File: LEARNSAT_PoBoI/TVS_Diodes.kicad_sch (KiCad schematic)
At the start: 4 parts

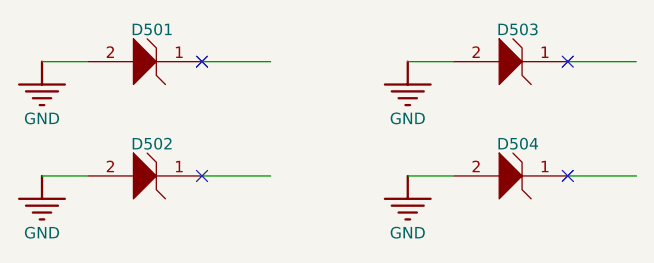
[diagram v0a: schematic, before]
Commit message: Add files via upload
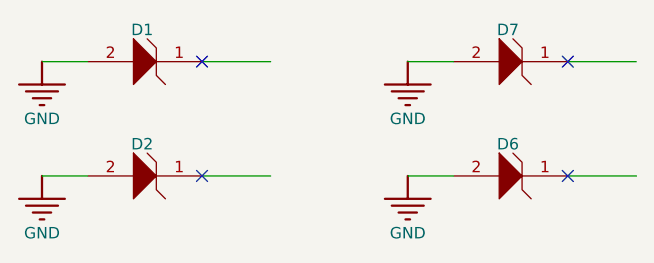
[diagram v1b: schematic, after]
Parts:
- D1: renamed from D501; footprint Diode_SMD:D_SOD-323 -> ONSC-SOD-323-2-477-02_V
- D2: renamed from D502; footprint Diode_SMD:D_SOD-323 -> ONSC-SOD-323-2-477-02_V
- D6: renamed from D504; footprint Diode_SMD:D_SOD-323 -> ONSC-SOD-323-2-477-02_V
- D7: renamed from D503; footprint Diode_SMD:D_SOD-323 -> ONSC-SOD-323-2-477-02_V
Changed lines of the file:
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@@
 		(on_board yes)
 		(dnp no)
-		(property "Reference" "#PWR0502"
+		(property "Reference" "#PWR?"
 			(at 58.42 111.76 0)
 			(effects
@@
 			(project ""
 				(path "/31302da5-a970-4b2b-aa05-afcd06cb9d09/9724113b-8f83-448f-99ae-c96db2fb53ca"
-					(reference "#PWR0502")
+					(reference "#PWR?")
 					(unit 1)
 				)
@@
 		(on_board yes)
 		(dnp no)
-		(property "Reference" "D503"
+		(property "Reference" "D7"
 			(at 108.966 96.266 0)
 			(effects
@@
 			)
 		)
-		(property "Footprint" "Diode_SMD:D_SOD-323"
+		(property "Footprint" "ONSC-SOD-323-2-477-02_V"
 			(at 111.76 101.6 0)
 			(effects
@@
 			(project ""
 				(path "/31302da5-a970-4b2b-aa05-afcd06cb9d09/9724113b-8f83-448f-99ae-c96db2fb53ca"
-					(reference "D503")
+					(reference "D7")
 					(unit 1)
 				)
@@
 		(on_board yes)
 		(dnp no)
-		(property "Reference" "#PWR0503"
+		(property "Reference" "#PWR?"
 			(at 99.06 99.06 0)
 			(effects
@@
 			(project ""
 				(path "/31302da5-a970-4b2b-aa05-afcd06cb9d09/9724113b-8f83-448f-99ae-c96db2fb53ca"
-					(reference "#PWR0503")
+					(reference "#PWR?")
 					(unit 1)
 				)
@@
 		(on_board yes)
 		(dnp no)
-		(property "Reference" "#PWR0504"
+		(property "Reference" "#PWR?"
 			(at 99.06 111.76 0)
 			(effects
@@
 			(project ""
 				(path "/31302da5-a970-4b2b-aa05-afcd06cb9d09/9724113b-8f83-448f-99ae-c96db2fb53ca"
-					(reference "#PWR0504")
+					(reference "#PWR?")
 					(unit 1)
 				)
@@
 		(on_board yes)
 		(dnp no)
-		(property "Reference" "D504"
+		(property "Reference" "D6"
 			(at 108.966 108.966 0)
 			(effects
@@
 			)
 		)
-		(property "Footprint" "Diode_SMD:D_SOD-323"
+		(property "Footprint" "ONSC-SOD-323-2-477-02_V"
 			(at 111.76 114.3 0)
 			(effects
@@
 			(project ""
 				(path "/31302da5-a970-4b2b-aa05-afcd06cb9d09/9724113b-8f83-448f-99ae-c96db2fb53ca"
-					(reference "D504")
+					(reference "D6")
 					(unit 1)
 				)
@@
 		(on_board yes)
 		(dnp no)
-		(property "Reference" "D501"
+		(property "Reference" "D1"
 			(at 68.326 96.266 0)
 			(effects
@@
 			)
 		)
-		(property "Footprint" "Diode_SMD:D_SOD-323"
+		(property "Footprint" "ONSC-SOD-323-2-477-02_V"
 			(at 71.12 101.6 0)
 			(effects
@@
 			(project ""
 				(path "/31302da5-a970-4b2b-aa05-afcd06cb9d09/9724113b-8f83-448f-99ae-c96db2fb53ca"
-					(reference "D501")
+					(reference "D1")
 					(unit 1)
 				)
@@
 		(on_board yes)
 		(dnp no)
-		(property "Reference" "D502"
+		(property "Reference" "D2"
 			(at 68.326 108.966 0)
 			(effects
@@
 			)
 		)
-		(property "Footprint" "Diode_SMD:D_SOD-323"
+		(property "Footprint" "ONSC-SOD-323-2-477-02_V"
 			(at 71.12 114.3 0)
 			(effects
@@
 			(project ""
 				(path "/31302da5-a970-4b2b-aa05-afcd06cb9d09/9724113b-8f83-448f-99ae-c96db2fb53ca"
-					(reference "D502")
+					(reference "D2")
 					(unit 1)
 				)
@@
 		(on_board yes)
 		(dnp no)
-		(property "Reference" "#PWR0501"
+		(property "Reference" "#PWR?"
 			(at 58.42 99.06 0)
 			(effects
@@
 			(project ""
 				(path "/31302da5-a970-4b2b-aa05-afcd06cb9d09/9724113b-8f83-448f-99ae-c96db2fb53ca"
-					(reference "#PWR0501")
+					(reference "#PWR?")
 					(unit 1)
 				)

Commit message: Added footprints
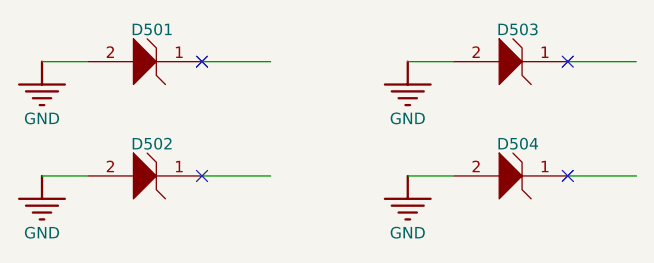
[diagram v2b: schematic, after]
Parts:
- D501: renamed from D1; footprint ONSC-SOD-323-2-477-02_V -> Diode_SMD:D_SOD-323
- D502: renamed from D2; footprint ONSC-SOD-323-2-477-02_V -> Diode_SMD:D_SOD-323
- D503: renamed from D7; footprint ONSC-SOD-323-2-477-02_V -> Diode_SMD:D_SOD-323
- D504: renamed from D6; footprint ONSC-SOD-323-2-477-02_V -> Diode_SMD:D_SOD-323
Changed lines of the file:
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@@
 		(on_board yes)
 		(dnp no)
-		(property "Reference" "#PWR?"
+		(property "Reference" "#PWR0502"
 			(at 58.42 111.76 0)
 			(effects
@@
 			(project ""
 				(path "/31302da5-a970-4b2b-aa05-afcd06cb9d09/9724113b-8f83-448f-99ae-c96db2fb53ca"
-					(reference "#PWR?")
+					(reference "#PWR0502")
 					(unit 1)
 				)
@@
 		(on_board yes)
 		(dnp no)
-		(property "Reference" "D7"
+		(property "Reference" "D503"
 			(at 108.966 96.266 0)
 			(effects
@@
 			)
 		)
-		(property "Footprint" "ONSC-SOD-323-2-477-02_V"
+		(property "Footprint" "Diode_SMD:D_SOD-323"
 			(at 111.76 101.6 0)
 			(effects
@@
 			(project ""
 				(path "/31302da5-a970-4b2b-aa05-afcd06cb9d09/9724113b-8f83-448f-99ae-c96db2fb53ca"
-					(reference "D7")
+					(reference "D503")
 					(unit 1)
 				)
@@
 		(on_board yes)
 		(dnp no)
-		(property "Reference" "#PWR?"
+		(property "Reference" "#PWR0503"
 			(at 99.06 99.06 0)
 			(effects
@@
 			(project ""
 				(path "/31302da5-a970-4b2b-aa05-afcd06cb9d09/9724113b-8f83-448f-99ae-c96db2fb53ca"
-					(reference "#PWR?")
+					(reference "#PWR0503")
 					(unit 1)
 				)
@@
 		(on_board yes)
 		(dnp no)
-		(property "Reference" "#PWR?"
+		(property "Reference" "#PWR0504"
 			(at 99.06 111.76 0)
 			(effects
@@
 			(project ""
 				(path "/31302da5-a970-4b2b-aa05-afcd06cb9d09/9724113b-8f83-448f-99ae-c96db2fb53ca"
-					(reference "#PWR?")
+					(reference "#PWR0504")
 					(unit 1)
 				)
@@
 		(on_board yes)
 		(dnp no)
-		(property "Reference" "D6"
+		(property "Reference" "D504"
 			(at 108.966 108.966 0)
 			(effects
@@
 			)
 		)
-		(property "Footprint" "ONSC-SOD-323-2-477-02_V"
+		(property "Footprint" "Diode_SMD:D_SOD-323"
 			(at 111.76 114.3 0)
 			(effects
@@
 			(project ""
 				(path "/31302da5-a970-4b2b-aa05-afcd06cb9d09/9724113b-8f83-448f-99ae-c96db2fb53ca"
-					(reference "D6")
+					(reference "D504")
 					(unit 1)
 				)
@@
 		(on_board yes)
 		(dnp no)
-		(property "Reference" "D1"
+		(property "Reference" "D501"
 			(at 68.326 96.266 0)
 			(effects
@@
 			)
 		)
-		(property "Footprint" "ONSC-SOD-323-2-477-02_V"
+		(property "Footprint" "Diode_SMD:D_SOD-323"
 			(at 71.12 101.6 0)
 			(effects
@@
 			(project ""
 				(path "/31302da5-a970-4b2b-aa05-afcd06cb9d09/9724113b-8f83-448f-99ae-c96db2fb53ca"
-					(reference "D1")
+					(reference "D501")
 					(unit 1)
 				)
@@
 		(on_board yes)
 		(dnp no)
-		(property "Reference" "D2"
+		(property "Reference" "D502"
 			(at 68.326 108.966 0)
 			(effects
@@
 			)
 		)
-		(property "Footprint" "ONSC-SOD-323-2-477-02_V"
+		(property "Footprint" "Diode_SMD:D_SOD-323"
 			(at 71.12 114.3 0)
 			(effects
@@
 			(project ""
 				(path "/31302da5-a970-4b2b-aa05-afcd06cb9d09/9724113b-8f83-448f-99ae-c96db2fb53ca"
-					(reference "D2")
+					(reference "D502")
 					(unit 1)
 				)
@@
 		(on_board yes)
 		(dnp no)
-		(property "Reference" "#PWR?"
+		(property "Reference" "#PWR0501"
 			(at 58.42 99.06 0)
 			(effects
@@
 			(project ""
 				(path "/31302da5-a970-4b2b-aa05-afcd06cb9d09/9724113b-8f83-448f-99ae-c96db2fb53ca"
-					(reference "#PWR?")
+					(reference "#PWR0501")
 					(unit 1)
 				)
